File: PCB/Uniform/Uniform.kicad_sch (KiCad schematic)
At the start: 156 parts, among them CON1 826629-5, CON2 Conn_01x03, U1 STM32L072KZT6

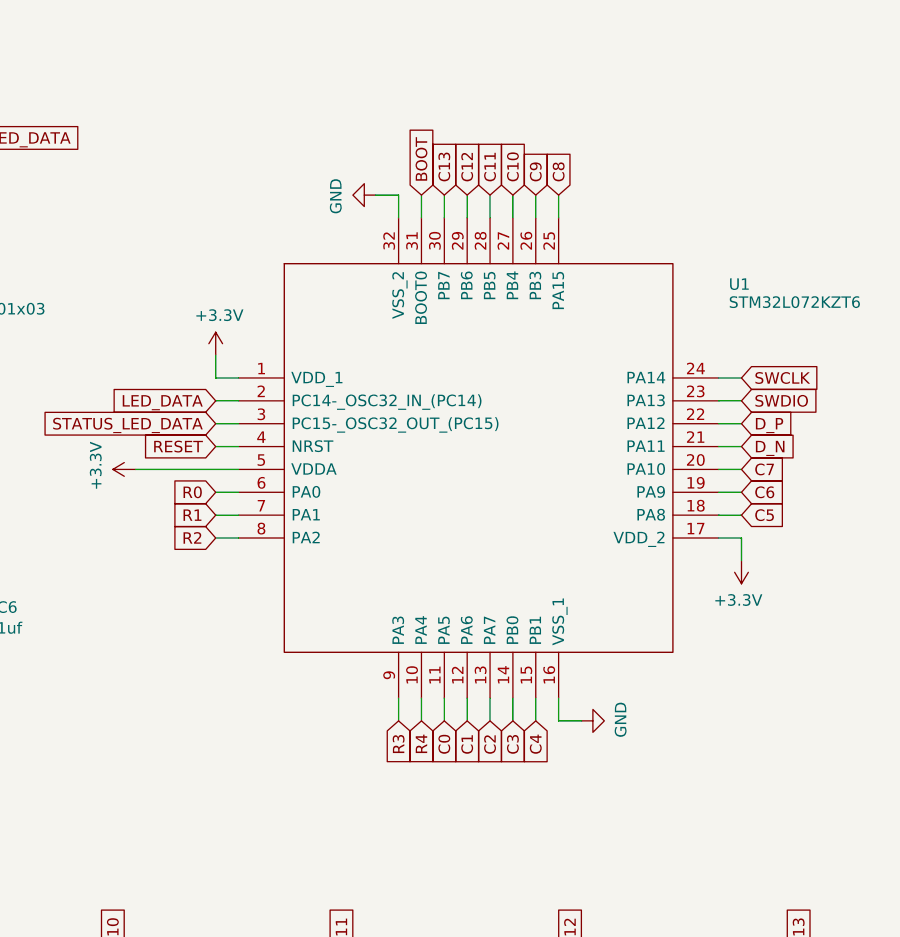
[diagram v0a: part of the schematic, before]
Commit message: about to attempt rotating the MCU
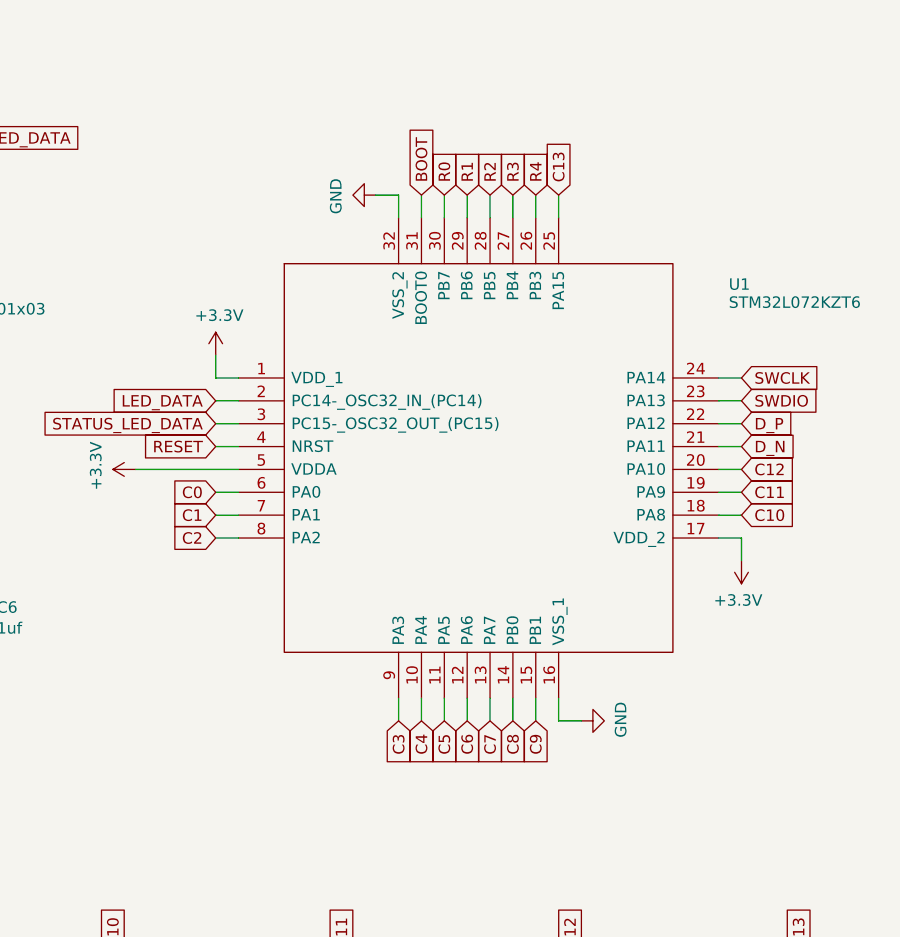
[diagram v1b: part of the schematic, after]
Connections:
- net C0: now also U1.6 (PA0); no longer U1.11 (PA5)
- net C1: now also U1.7 (PA1); no longer U1.12 (PA6)
- net C10: now also U1.18 (PA8); no longer U1.27 (PB4)
- net C11: now also U1.19 (PA9); no longer U1.28 (PB5)
- net C12: now also U1.20 (PA10); no longer U1.29 (PB6)
- net C13: now also U1.25 (PA15); no longer U1.30 (PB7)
- net C2: now also U1.8 (PA2); no longer U1.13 (PA7)
- net C3: now also U1.9 (PA3); no longer U1.14 (PB0)
- net C4: now also U1.10 (PA4); no longer U1.15 (PB1)
- net C5: now also U1.11 (PA5); no longer U1.18 (PA8)
- net C6: now also U1.12 (PA6); no longer U1.19 (PA9)
- net C7: now also U1.13 (PA7); no longer U1.20 (PA10)
- net C8: now also U1.14 (PB0); no longer U1.25 (PA15)
- net C9: now also U1.15 (PB1); no longer U1.26 (PB3)
- net R0: now also U1.30 (PB7); no longer U1.6 (PA0)
- net R1: now also U1.29 (PB6); no longer U1.7 (PA1)
- net R2: now also U1.28 (PB5); no longer U1.8 (PA2)
- net R3: now also U1.27 (PB4); no longer U1.9 (PA3)
- net R4: now also U1.26 (PB3); no longer U1.10 (PA4)
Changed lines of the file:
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@@
     )
   )
-  (global_label "C0" (shape input) (at 349.25 92.71 270) (fields_autoplaced)
-    (effects (font (size 1.27 1.27)) (justify right))
-    (property "Intersheet References" "${INTERSHEET_REFS}" (id 0) (at 0 0 0)
-      (effects (font (size 1.27 1.27)) hide)
-    )
-  )
-  (global_label "C9" (shape input) (at 359.41 34.29 90) (fields_autoplaced)
-    (effects (font (size 1.27 1.27)) (justify left))
-    (property "Intersheet References" "${INTERSHEET_REFS}" (id 0) (at 0 0 0)
+  (global_label "C0" (shape input) (at 323.85 67.31 180) (fields_autoplaced)
+    (effects (font (size 1.27 1.27)) (justify right))
+    (property "Intersheet References" "${INTERSHEET_REFS}" (id 0) (at 416.56 -281.94 0)
+      (effects (font (size 1.27 1.27)) hide)
+    )
+  )
+  (global_label "C9" (shape input) (at 359.41 92.71 270) (fields_autoplaced)
+    (effects (font (size 1.27 1.27)) (justify right))
+    (property "Intersheet References" "${INTERSHEET_REFS}" (id 0) (at 718.82 127 0)
       (effects (font (size 1.27 1.27)) hide)
     )
@@
     )
   )
-  (global_label "R1" (shape input) (at 323.85 69.85 180) (fields_autoplaced)
-    (effects (font (size 1.27 1.27)) (justify right))
-    (property "Intersheet References" "${INTERSHEET_REFS}" (id 0) (at 0 0 0)
+  (global_label "R1" (shape input) (at 351.79 34.29 90) (fields_autoplaced)
+    (effects (font (size 1.27 1.27)) (justify left))
+    (property "Intersheet References" "${INTERSHEET_REFS}" (id 0) (at 421.64 -289.56 0)
       (effects (font (size 1.27 1.27)) hide)
     )
@@
     )
   )
-  (global_label "R2" (shape input) (at 323.85 72.39 180) (fields_autoplaced)
-    (effects (font (size 1.27 1.27)) (justify right))
-    (property "Intersheet References" "${INTERSHEET_REFS}" (id 0) (at 0 0 0)
-      (effects (font (size 1.27 1.27)) hide)
-    )
-  )
-  (global_label "C7" (shape input) (at 382.27 64.77 0) (fields_autoplaced)
-    (effects (font (size 1.27 1.27)) (justify left))
-    (property "Intersheet References" "${INTERSHEET_REFS}" (id 0) (at 0 0 0)
+  (global_label "R2" (shape input) (at 354.33 34.29 90) (fields_autoplaced)
+    (effects (font (size 1.27 1.27)) (justify left))
+    (property "Intersheet References" "${INTERSHEET_REFS}" (id 0) (at 426.72 -289.56 0)
+      (effects (font (size 1.27 1.27)) hide)
+    )
+  )
+  (global_label "C7" (shape input) (at 354.33 92.71 270) (fields_autoplaced)
+    (effects (font (size 1.27 1.27)) (justify right))
+    (property "Intersheet References" "${INTERSHEET_REFS}" (id 0) (at 419.1 -289.56 0)
       (effects (font (size 1.27 1.27)) hide)
     )
@@
     )
   )
-  (global_label "R0" (shape input) (at 323.85 67.31 180) (fields_autoplaced)
-    (effects (font (size 1.27 1.27)) (justify right))
-    (property "Intersheet References" "${INTERSHEET_REFS}" (id 0) (at 0 0 0)
-      (effects (font (size 1.27 1.27)) hide)
-    )
-  )
-  (global_label "C3" (shape input) (at 356.87 92.71 270) (fields_autoplaced)
-    (effects (font (size 1.27 1.27)) (justify right))
-    (property "Intersheet References" "${INTERSHEET_REFS}" (id 0) (at 0 0 0)
+  (global_label "R0" (shape input) (at 349.25 34.29 90) (fields_autoplaced)
+    (effects (font (size 1.27 1.27)) (justify left))
+    (property "Intersheet References" "${INTERSHEET_REFS}" (id 0) (at 416.56 -289.56 0)
+      (effects (font (size 1.27 1.27)) hide)
+    )
+  )
+  (global_label "C3" (shape input) (at 344.17 92.71 270) (fields_autoplaced)
+    (effects (font (size 1.27 1.27)) (justify right))
+    (property "Intersheet References" "${INTERSHEET_REFS}" (id 0) (at -12.7 0 0)
       (effects (font (size 1.27 1.27)) hide)
     )
@@
     )
   )
-  (global_label "C5" (shape input) (at 382.27 69.85 0) (fields_autoplaced)
-    (effects (font (size 1.27 1.27)) (justify left))
-    (property "Intersheet References" "${INTERSHEET_REFS}" (id 0) (at 0 0 0)
+  (global_label "C5" (shape input) (at 349.25 92.71 270) (fields_autoplaced)
+    (effects (font (size 1.27 1.27)) (justify right))
+    (property "Intersheet References" "${INTERSHEET_REFS}" (id 0) (at 419.1 -289.56 0)
       (effects (font (size 1.27 1.27)) hide)
     )
@@
     )
   )
-  (global_label "R3" (shape input) (at 344.17 92.71 270) (fields_autoplaced)
-    (effects (font (size 1.27 1.27)) (justify right))
-    (property "Intersheet References" "${INTERSHEET_REFS}" (id 0) (at 0 0 0)
-      (effects (font (size 1.27 1.27)) hide)
-    )
-  )
-  (global_label "C4" (shape input) (at 359.41 92.71 270) (fields_autoplaced)
-    (effects (font (size 1.27 1.27)) (justify right))
-    (property "Intersheet References" "${INTERSHEET_REFS}" (id 0) (at 0 0 0)
+  (global_label "R3" (shape input) (at 356.87 34.29 90) (fields_autoplaced)
+    (effects (font (size 1.27 1.27)) (justify left))
+    (property "Intersheet References" "${INTERSHEET_REFS}" (id 0) (at 701.04 127 0)
+      (effects (font (size 1.27 1.27)) hide)
+    )
+  )
+  (global_label "C4" (shape input) (at 346.71 92.71 270) (fields_autoplaced)
+    (effects (font (size 1.27 1.27)) (justify right))
+    (property "Intersheet References" "${INTERSHEET_REFS}" (id 0) (at -12.7 0 0)
       (effects (font (size 1.27 1.27)) hide)
     )
@@
     )
   )
-  (global_label "R4" (shape input) (at 346.71 92.71 270) (fields_autoplaced)
-    (effects (font (size 1.27 1.27)) (justify right))
-    (property "Intersheet References" "${INTERSHEET_REFS}" (id 0) (at 0 0 0)
+  (global_label "R4" (shape input) (at 359.41 34.29 90) (fields_autoplaced)
+    (effects (font (size 1.27 1.27)) (justify left))
+    (property "Intersheet References" "${INTERSHEET_REFS}" (id 0) (at 706.12 127 0)
       (effects (font (size 1.27 1.27)) hide)
     )
@@
     )
   )
-  (global_label "C13" (shape input) (at 349.25 34.29 90) (fields_autoplaced)
-    (effects (font (size 1.27 1.27)) (justify left))
-    (property "Intersheet References" "${INTERSHEET_REFS}" (id 0) (at 0 0 0)
+  (global_label "C13" (shape input) (at 361.95 34.29 90) (fields_autoplaced)
+    (effects (font (size 1.27 1.27)) (justify left))
+    (property "Intersheet References" "${INTERSHEET_REFS}" (id 0) (at 12.7 0 0)
       (effects (font (size 1.27 1.27)) hide)
     )
@@
     )
   )
-  (global_label "C11" (shape input) (at 354.33 34.29 90) (fields_autoplaced)
-    (effects (font (size 1.27 1.27)) (justify left))
-    (property "Intersheet References" "${INTERSHEET_REFS}" (id 0) (at 0 0 0)
+  (global_label "C11" (shape input) (at 382.27 67.31 0) (fields_autoplaced)
+    (effects (font (size 1.27 1.27)) (justify left))
+    (property "Intersheet References" "${INTERSHEET_REFS}" (id 0) (at 416.56 -287.02 0)
       (effects (font (size 1.27 1.27)) hide)
     )
@@
     )
   )
-  (global_label "C8" (shape input) (at 361.95 34.29 90) (fields_autoplaced)
-    (effects (font (size 1.27 1.27)) (justify left))
-    (property "Intersheet References" "${INTERSHEET_REFS}" (id 0) (at 0 0 0)
-      (effects (font (size 1.27 1.27)) hide)
-    )
-  )
-  (global_label "C6" (shape input) (at 382.27 67.31 0) (fields_autoplaced)
-    (effects (font (size 1.27 1.27)) (justify left))
-    (property "Intersheet References" "${INTERSHEET_REFS}" (id 0) (at 0 0 0)
-      (effects (font (size 1.27 1.27)) hide)
-    )
-  )
-  (global_label "C2" (shape input) (at 354.33 92.71 270) (fields_autoplaced)
-    (effects (font (size 1.27 1.27)) (justify right))
-    (property "Intersheet References" "${INTERSHEET_REFS}" (id 0) (at 0 0 0)
+  (global_label "C8" (shape input) (at 356.87 92.71 270) (fields_autoplaced)
+    (effects (font (size 1.27 1.27)) (justify right))
+    (property "Intersheet References" "${INTERSHEET_REFS}" (id 0) (at 718.82 127 0)
+      (effects (font (size 1.27 1.27)) hide)
+    )
+  )
+  (global_label "C6" (shape input) (at 351.79 92.71 270) (fields_autoplaced)
+    (effects (font (size 1.27 1.27)) (justify right))
+    (property "Intersheet References" "${INTERSHEET_REFS}" (id 0) (at 419.1 -289.56 0)
+      (effects (font (size 1.27 1.27)) hide)
+    )
+  )
+  (global_label "C2" (shape input) (at 323.85 72.39 180) (fields_autoplaced)
+    (effects (font (size 1.27 1.27)) (justify right))
+    (property "Intersheet References" "${INTERSHEET_REFS}" (id 0) (at 416.56 -281.94 0)
       (effects (font (size 1.27 1.27)) hide)
     )
@@
     )
   )
-  (global_label "C1" (shape input) (at 351.79 92.71 270) (fields_autoplaced)
-    (effects (font (size 1.27 1.27)) (justify right))
-    (property "Intersheet References" "${INTERSHEET_REFS}" (id 0) (at 0 0 0)
-      (effects (font (size 1.27 1.27)) hide)
-    )
-  )
-  (global_label "C10" (shape input) (at 356.87 34.29 90) (fields_autoplaced)
-    (effects (font (size 1.27 1.27)) (justify left))
-    (property "Intersheet References" "${INTERSHEET_REFS}" (id 0) (at 0 0 0)
+  (global_label "C1" (shape input) (at 323.85 69.85 180) (fields_autoplaced)
+    (effects (font (size 1.27 1.27)) (justify right))
+    (property "Intersheet References" "${INTERSHEET_REFS}" (id 0) (at 416.56 -281.94 0)
+      (effects (font (size 1.27 1.27)) hide)
+    )
+  )
+  (global_label "C10" (shape input) (at 382.27 69.85 0) (fields_autoplaced)
+    (effects (font (size 1.27 1.27)) (justify left))
+    (property "Intersheet References" "${INTERSHEET_REFS}" (id 0) (at 416.56 -287.02 0)
       (effects (font (size 1.27 1.27)) hide)
     )
@@
     )
   )
-  (global_label "C12" (shape input) (at 351.79 34.29 90) (fields_autoplaced)
-    (effects (font (size 1.27 1.27)) (justify left))
-    (property "Intersheet References" "${INTERSHEET_REFS}" (id 0) (at 0 0 0)
-      (effects (font (size 1.27 1.27)) hide)
-    )
+  (global_label "C12" (shape input) (at 382.27 64.77 0) (fields_autoplaced)
+    (effects (font (size 1.27 1.27)) (justify left))
+    (property "Intersheet References" "${INTERSHEET_REFS}" (id 0) (at 416.56 -287.02 0)
+      (effects (font (size 1.27 1.27)) hide)
+    )

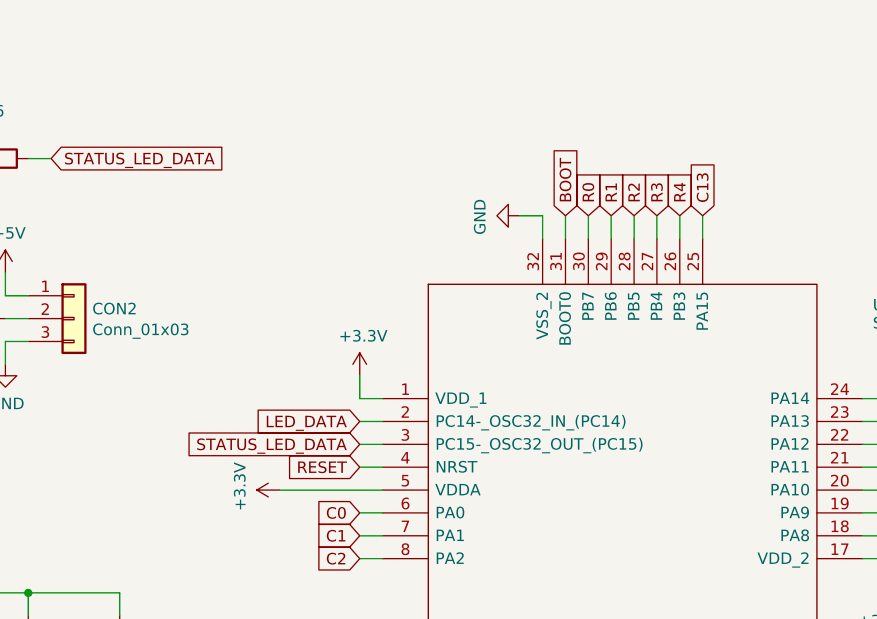
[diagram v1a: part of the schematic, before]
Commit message: PCB first pass complete
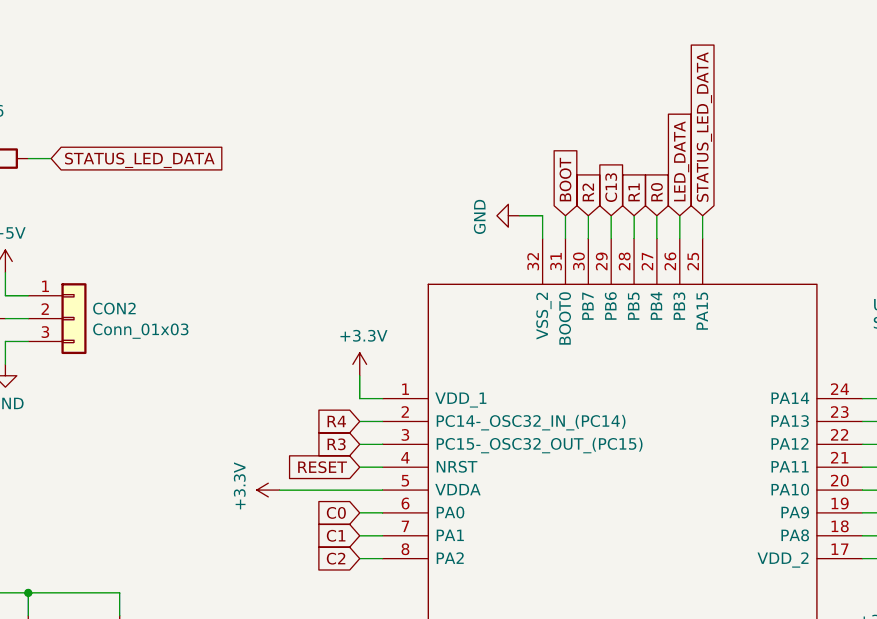
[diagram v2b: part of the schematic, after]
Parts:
- LED1: footprint LED_THT:LED_D5.0mm_Clear -> LED_THT:LED_D3.0mm_Clear
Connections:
- net C13: now also U1.29 (PB6); no longer U1.25 (PA15)
- net LED_DATA: now also U1.26 (PB3); no longer U1.2 (PC14-_OSC32_IN_(PC14))
- net R0: now also U1.27 (PB4); no longer U1.30 (PB7)
- net R1: now also U1.28 (PB5); no longer U1.29 (PB6)
- net R2: now also U1.30 (PB7); no longer U1.28 (PB5)
- net R3: now also U1.3 (PC15-_OSC32_OUT_(PC15)); no longer U1.27 (PB4)
- net R4: now also U1.2 (PC14-_OSC32_IN_(PC14)); no longer U1.26 (PB3)
- net STATUS_LED_DATA: now also U1.25 (PA15); no longer U1.3 (PC15-_OSC32_OUT_(PC15))
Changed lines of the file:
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@@
     )
   )
-  (global_label "R1" (shape input) (at 351.79 34.29 90) (fields_autoplaced)
+  (global_label "R1" (shape input) (at 354.33 34.29 90) (fields_autoplaced)
     (effects (font (size 1.27 1.27)) (justify left))
-    (property "Intersheet References" "${INTERSHEET_REFS}" (id 0) (at 421.64 -289.56 0)
+    (property "Intersheet References" "${INTERSHEET_REFS}" (id 0) (at 424.18 -289.56 0)
       (effects (font (size 1.27 1.27)) hide)
     )
@@
     )
   )
-  (global_label "STATUS_LED_DATA" (shape input) (at 323.85 59.69 180) (fields_autoplaced)
-    (effects (font (size 1.27 1.27)) (justify right))
-    (property "Intersheet References" "${INTERSHEET_REFS}" (id 0) (at 0 0 0)
+  (global_label "STATUS_LED_DATA" (shape input) (at 361.95 34.29 90) (fields_autoplaced)
+    (effects (font (size 1.27 1.27)) (justify left))
+    (property "Intersheet References" "${INTERSHEET_REFS}" (id 0) (at 421.64 -289.56 0)
       (effects (font (size 1.27 1.27)) hide)
     )
@@
     )
   )
-  (global_label "R2" (shape input) (at 354.33 34.29 90) (fields_autoplaced)
+  (global_label "R2" (shape input) (at 349.25 34.29 90) (fields_autoplaced)
     (effects (font (size 1.27 1.27)) (justify left))
-    (property "Intersheet References" "${INTERSHEET_REFS}" (id 0) (at 426.72 -289.56 0)
+    (property "Intersheet References" "${INTERSHEET_REFS}" (id 0) (at 421.64 -289.56 0)
       (effects (font (size 1.27 1.27)) hide)
     )
@@
     )
   )
-  (global_label "R0" (shape input) (at 349.25 34.29 90) (fields_autoplaced)
+  (global_label "R0" (shape input) (at 356.87 34.29 90) (fields_autoplaced)
     (effects (font (size 1.27 1.27)) (justify left))
-    (property "Intersheet References" "${INTERSHEET_REFS}" (id 0) (at 416.56 -289.56 0)
+    (property "Intersheet References" "${INTERSHEET_REFS}" (id 0) (at 424.18 -289.56 0)
       (effects (font (size 1.27 1.27)) hide)
     )
@@
     )
   )
-  (global_label "R3" (shape input) (at 356.87 34.29 90) (fields_autoplaced)
-    (effects (font (size 1.27 1.27)) (justify left))
-    (property "Intersheet References" "${INTERSHEET_REFS}" (id 0) (at 701.04 127 0)
+  (global_label "R3" (shape input) (at 323.85 59.69 180) (fields_autoplaced)
+    (effects (font (size 1.27 1.27)) (justify right))
+    (property "Intersheet References" "${INTERSHEET_REFS}" (id 0) (at 416.56 -284.48 0)
       (effects (font (size 1.27 1.27)) hide)
     )
@@
     )
   )
-  (global_label "R4" (shape input) (at 359.41 34.29 90) (fields_autoplaced)
-    (effects (font (size 1.27 1.27)) (justify left))
-    (property "Intersheet References" "${INTERSHEET_REFS}" (id 0) (at 706.12 127 0)
+  (global_label "R4" (shape input) (at 323.85 57.15 180) (fields_autoplaced)
+    (effects (font (size 1.27 1.27)) (justify right))
+    (property "Intersheet References" "${INTERSHEET_REFS}" (id 0) (at 416.56 -289.56 0)
       (effects (font (size 1.27 1.27)) hide)
     )
@@
     )
   )
-  (global_label "C13" (shape input) (at 361.95 34.29 90) (fields_autoplaced)
+  (global_label "C13" (shape input) (at 351.79 34.29 90) (fields_autoplaced)
     (effects (font (size 1.27 1.27)) (justify left))
-    (property "Intersheet References" "${INTERSHEET_REFS}" (id 0) (at 12.7 0 0)
+    (property "Intersheet References" "${INTERSHEET_REFS}" (id 0) (at 2.54 0 0)
       (effects (font (size 1.27 1.27)) hide)
     )
@@
     )
   )
-  (global_label "LED_DATA" (shape input) (at 323.85 57.15 180) (fields_autoplaced)
-    (effects (font (size 1.27 1.27)) (justify right))
-    (property "Intersheet References" "${INTERSHEET_REFS}" (id 0) (at 0 0 0)
+  (global_label "LED_DATA" (shape input) (at 359.41 34.29 90) (fields_autoplaced)
+    (effects (font (size 1.27 1.27)) (justify left))
+    (property "Intersheet References" "${INTERSHEET_REFS}" (id 0) (at 416.56 -289.56 0)
       (effects (font (size 1.27 1.27)) hide)
     )
@@
     (property "Reference" "LED1" (id 0) (at 272.8722 22.4282 0))
     (property "Value" "LED" (id 1) (at 272.8722 24.7396 0))
-    (property "Footprint" "LED_THT:LED_D5.0mm_Clear" (id 2) (at 273.05 27.94 0)
+    (property "Footprint" "LED_THT:LED_D3.0mm_Clear" (id 2) (at 273.05 27.94 0)
       (effects (font (size 1.27 1.27)) hide)
     )
@@
     )
     (path "/00000000-0000-0000-0000-0000646a674a"
-      (reference "LED1") (unit 1) (value "LED") (footprint "LED_THT:LED_D5.0mm_Clear")
+      (reference "LED1") (unit 1) (value "LED") (footprint "LED_THT:LED_D3.0mm_Clear")
     )
     (path "/00000000-0000-0000-0000-000063eb21f8"
